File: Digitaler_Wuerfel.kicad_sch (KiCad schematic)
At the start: 40 parts, among them J1 Conn_01x03_Pin, J2 Conn_02x03_Odd_Even, SW1 SW_Push, SW2 SW_Push, SW3 SW_Push, SW4 SW_SPST, U1 74HC595, U2 74HC595, U3 ATmega328PB-A, U4 LM7805_TO220

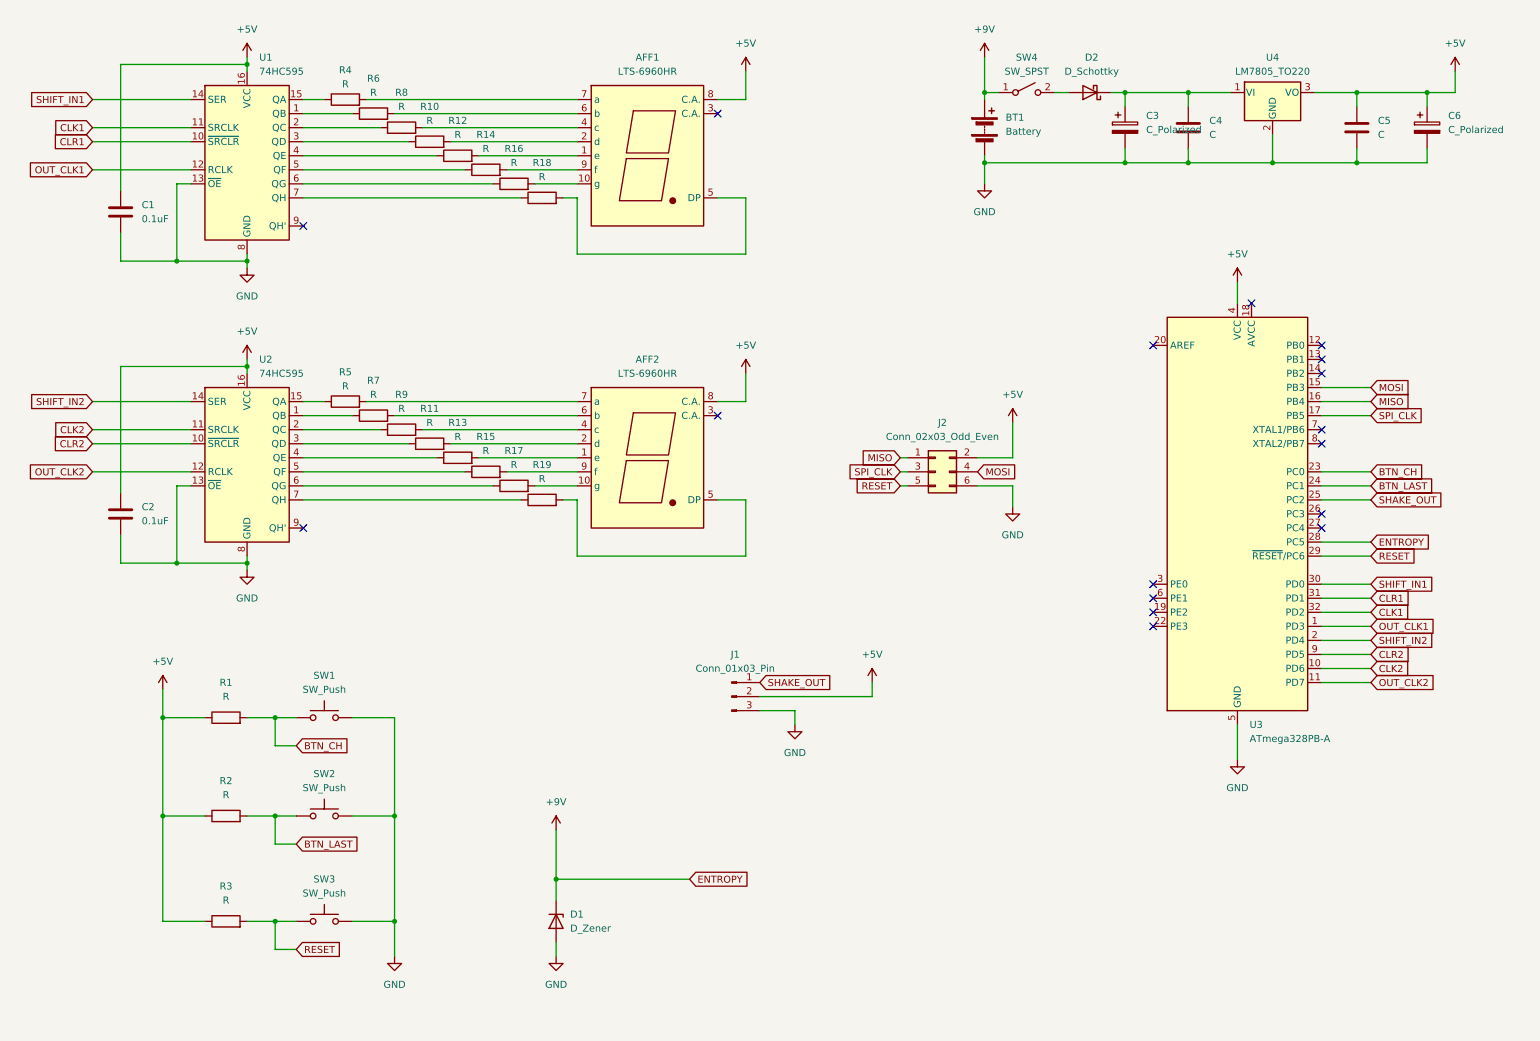
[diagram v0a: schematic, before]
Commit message: Started tracing
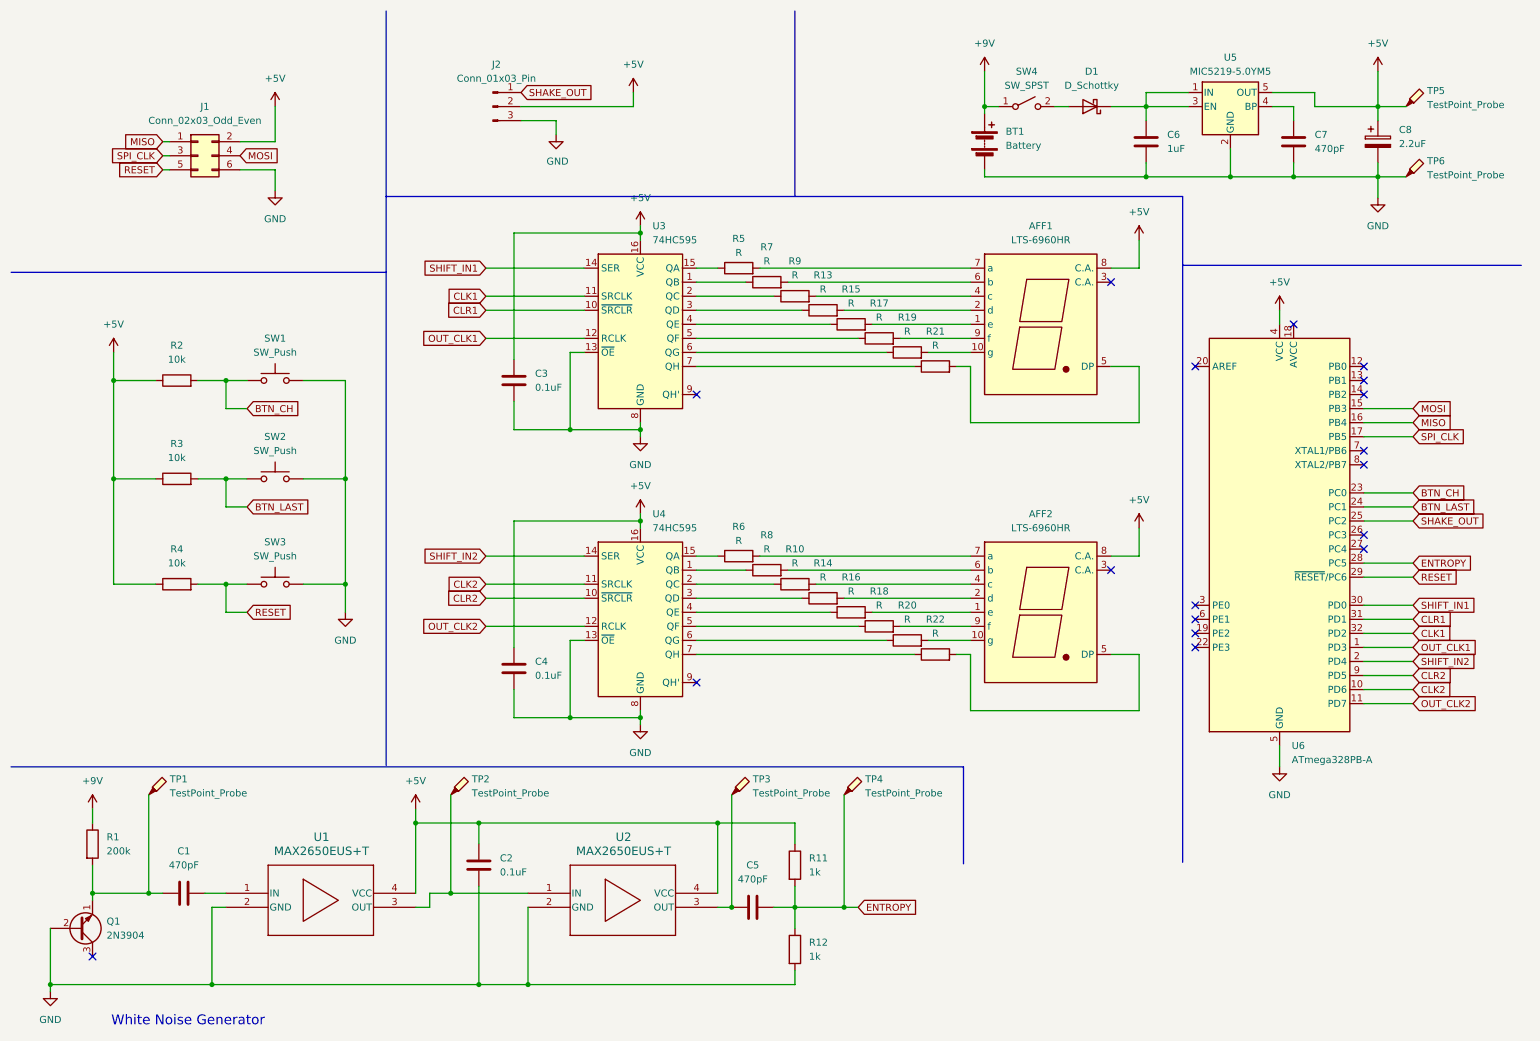
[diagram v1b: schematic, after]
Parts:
- removed C3, C6: C_Polarized, symbol Device:C_Polarized
- removed D1: D_Zener, symbol Device:D_Zener
- removed U4: LM7805_TO220, Package_TO_SOT_THT:TO-220-3_Horizontal_TabDown, symbol Regulator_Linear:LM7805_TO220
- added C1, C7: 470pF, Capacitor_SMD:C_0805_2012Metric_Pad1.18x1.45mm_HandSolder, symbol Device:C
- added C2: 0.1uF, Capacitor_SMD:C_0805_2012Metric_Pad1.18x1.45mm_HandSolder, symbol Device:C
- added C8: 2.2uF, Capacitor_Tantalum_SMD:CP_EIA-3528-21_Kemet-B_Pad1.50x2.35mm_HandSolder, symbol Device:C_Polarized
- added Q1: 2N3904, Package_TO_SOT_THT:TO-92_Inline, symbol Transistor_BJT:2N3904
- added R1: 200k, Resistor_SMD:R_0805_2012Metric_Pad1.20x1.40mm_HandSolder, symbol Device:R
- added R11, R12: 1k, Resistor_SMD:R_0805_2012Metric_Pad1.20x1.40mm_HandSolder, symbol Device:R
- added TP1, TP2, TP3, TP4, TP5, TP6: TestPoint_Probe, TestPoint:TestPoint_Pad_D2.0mm, symbol Connector:TestPoint_Probe
- added U1, U2: MAX2650EUS+T, MAX2650EUS+T:21-0052F_MXM, symbol MAX2650EUS+T:MAX2650EUS+T
- added U5: MIC5219-5.0YM5, Package_TO_SOT_SMD:SOT-23-5, symbol Regulator_Linear:MIC5219-5.0YM5
- C5: value C -> 470pF
- C6: renamed from C4; value C -> 1uF
- D1: renamed from D2; footprint (none) -> Diode_SMD:D_SOD-323_HandSoldering
- R2: renamed from R1; value R -> 10k
- R3: renamed from R2; value R -> 10k
- R4: renamed from R3; value R -> 10k
- SW1, SW2: footprint (none) -> Button_Switch_THT:SW_PUSH-12mm_Wuerth-430476085716
- SW3: footprint (none) -> Button_Switch_THT:SW_PUSH_6mm_H5mm
- SW4: footprint (none) -> Button_Switch_THT:SW_E-Switch_EG1271_SPDT
- renumbered C1 to C3, C2 to C4, J2 to J1, J1 to J2, R9 to R10, R10 to R13, R11 to R14, R12 to R15, R13 to R16, R14 to R17, R15 to R18, R16 to R19, R17 to R20, R18 to R21, R19 to R22, R4 to R5, R5 to R6, R6 to R7, R7 to R8, R8 to R9, U1 to U3, U2 to U4, U3 to U6
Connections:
- net +5V: now also C2.2, C8.1, R11.1, TP5.1, U1.4 (VCC), U2.4 (VCC), U5.5 (OUT); no longer C5.1
- net +9V: now also R1.1; no longer U6.28 (PC5)
- net GND: now also C2.1, C7.2, C8.2, Q1.2 (B), R12.2, TP6.1, U1.2 (GND), U2.2 (GND), U5.2 (GND); no longer C5.2
- net at C6.1, D1.1 (K): now also U5.1 (IN), U5.3 (EN)
- new net: C1.2, U1.1 (IN)
- new net: TP2.1, U1.3 (OUT), U2.1 (IN)
- new net: C1.1, Q1.1 (E), R1.2, TP1.1
- new net: C7.1, U5.4 (BP)
- new net: C5.1, TP3.1, U2.3 (OUT)
- new net ENTROPY: C5.2, R11.2, R12.1, TP4.1, U6.28 (PC5)
- no-connect marks 17 -> 18
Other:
- note added: "White Noise Generator"
- moved on the sheet: AFF1, AFF2, BT1, C3, C4, C6, D1, J1, J2, R10, R13, R14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
